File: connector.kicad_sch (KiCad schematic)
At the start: 4 parts, among them J3 Screw_Terminal_01x04

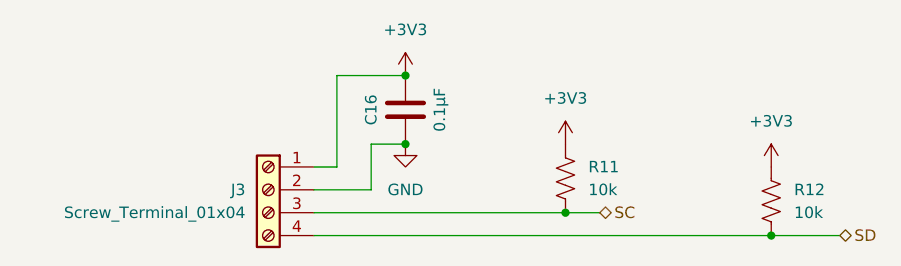
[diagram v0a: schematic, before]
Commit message: roughly complete, no errors or warnings.
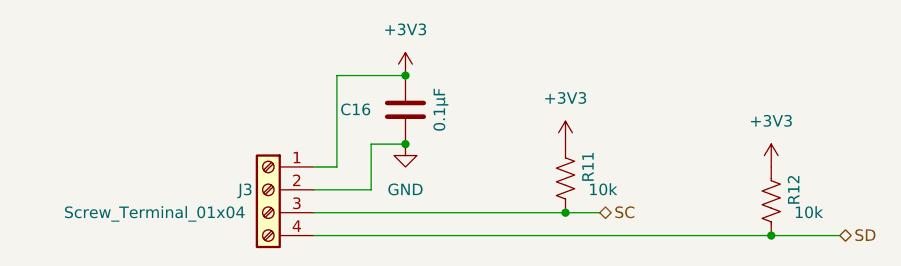
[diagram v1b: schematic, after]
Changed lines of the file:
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@@
 		(fields_autoplaced yes)
 		(property "Reference" "R11"
-			(at 105.41 41.91 0)
-			(effects
-				(font
-					(size 1.27 1.27)
-				)
-				(justify left)
+			(at 105.41 41.91 90)
+			(effects
+				(font
+					(size 1.27 1.27)
+				)
 			)
 		)
@@
 		(fields_autoplaced yes)
 		(property "Reference" "R12"
-			(at 128.27 44.45 0)
-			(effects
-				(font
-					(size 1.27 1.27)
-				)
-				(justify left)
+			(at 128.27 44.45 90)
+			(effects
+				(font
+					(size 1.27 1.27)
+				)
 			)
 		)
@@
 		(dnp no)
 		(property "Reference" "C16"
-			(at 81.28 35.56 90)
-			(effects
-				(font
-					(size 1.27 1.27)
-				)
+			(at 81.28 35.56 0)
+			(effects
+				(font
+					(size 1.27 1.27)
+				)
+				(justify left)
 			)
 		)
@@
 					(size 1.27 1.27)
 				)
-				(justify left)
-			)
-		)
+			)
+		)
